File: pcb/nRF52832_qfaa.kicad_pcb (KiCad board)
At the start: 4 copper layers, 41 x 12 mm, 58 parts, among them J2 Conn_02x05_Odd_Even, U1 NRF52832, U2 W25Q32JVZP, U3 TLV75533PDBVR, U4 BQ24078RGTR, X1 32.768kHz, X2 32MHz

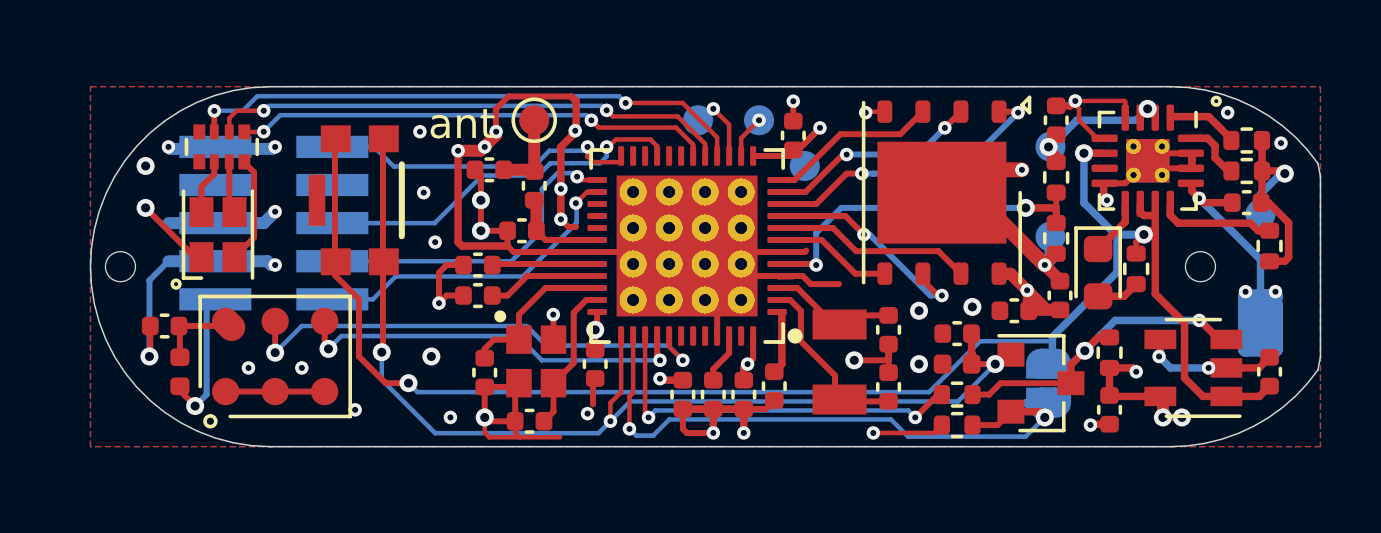
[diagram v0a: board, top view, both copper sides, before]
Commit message: [pcb] v1.2 schematics and PCB, start of the fixture
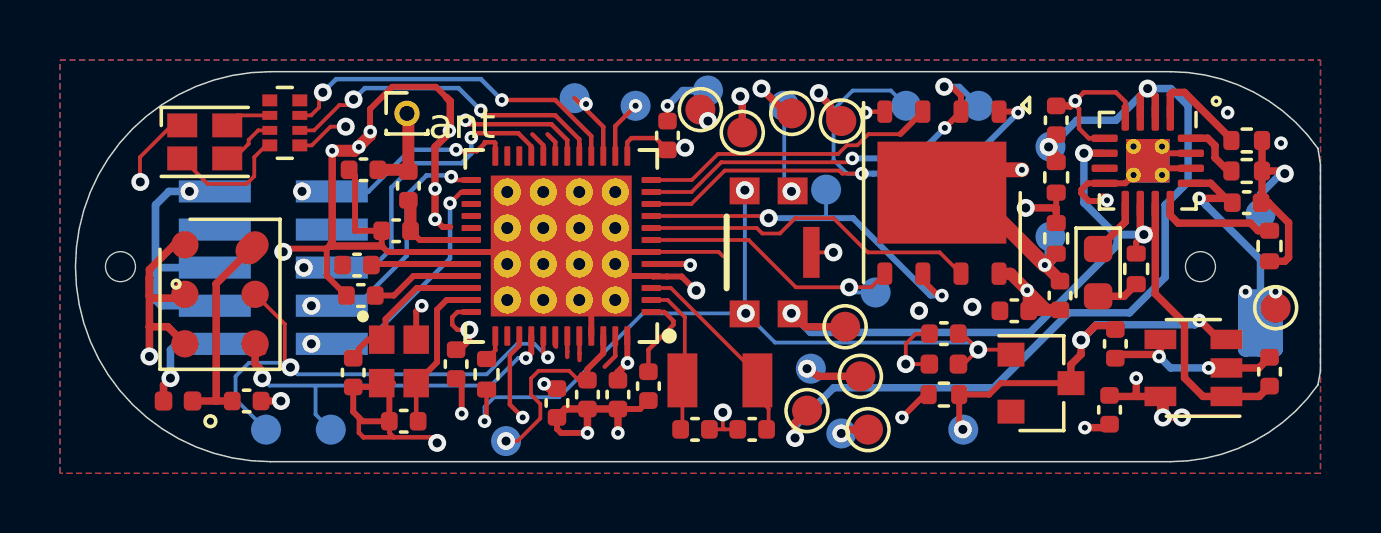
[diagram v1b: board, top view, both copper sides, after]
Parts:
- removed JP1: Jumper_2_Open, Jumper:SolderJumper-2_P1.3mm_Open_RoundedPad1.0x1.5mm
- removed R2: 100K, Resistor_SMD:R_0402_1005Metric
- removed R4: 10K, Resistor_SMD:R_0402_1005Metric
- removed TP5: Antenna, TestPoint:TestPoint_Pad_D1.0mm
- added C23: 100pF, Capacitor_SMD:C_0402_1005Metric, F.Cu at (64.1, 37.9)
- added J1: Conn_01x01_Female, Connector_PinHeader_1.00mm:PinHeader_1x01_P1.00mm_Vertical, F.Cu at (40.5, 30.2)
- added R13: 330, Resistor_SMD:R_0402_1005Metric, F.Cu at (43.2, 38.9)
- added TP10: TestPoint, TestPoint:TestPoint_Pad_D1.0mm, B.Cu at (35.8, 40.8)
- added TP11: TestPoint, TestPoint:TestPoint_Pad_D1.0mm, B.Cu at (43.8, 41.1)
- added TP12: TestPoint, TestPoint:TestPoint_Pad_D1.0mm, B.Cu at (56.1, 36.2)
- added TP13: TestPoint, TestPoint:TestPoint_Pad_D1.0mm, B.Cu at (57.1, 30.0)
- added TP14: TestPoint, TestPoint:TestPoint_Pad_D1.0mm, B.Cu at (59.6, 30.0)
- added TP15: TestPoint, TestPoint:TestPoint_Pad_D1.0mm, B.Cu at (54.5, 32.8)
- added TP16: TestPoint, TestPoint:TestPoint_Pad_D1.0mm, B.Cu at (59.1, 40.8)
- added TP17: TestPoint, TestPoint:TestPoint_Pad_D1.0mm, B.Cu at (54.0, 38.7)
- added TP18: TestPoint, TestPoint:TestPoint_Pad_D1.0mm, B.Cu at (53.1, 30.0)
- added TP19: TestPoint, TestPoint:TestPoint_Pad_D1.0mm, B.Cu at (55.0, 40.9)
- added TP20: TestPoint, TestPoint:TestPoint_Pad_D1.0mm, F.Cu at (50.3, 30.1)
- added TP21: TestPoint, TestPoint:TestPoint_Pad_D1.0mm, F.Cu at (55.0, 30.5)
- added TP22: TestPoint, TestPoint:TestPoint_Pad_D1.0mm, F.Cu at (51.7, 30.9)
- added TP23: TestPoint, TestPoint:TestPoint_Pad_D1.0mm, F.Cu at (53.3, 30.2)
- added TP24: TestPoint, TestPoint:TestPoint_Pad_D1.0mm, F.Cu at (55.1, 37.3)
- added TP25: TestPoint, TestPoint:TestPoint_Pad_D1.0mm, F.Cu at (55.6, 39.0)
- added TP26: TestPoint, TestPoint:TestPoint_Pad_D1.0mm, F.Cu at (69.5, 36.7)
- added TP27: TestPoint, TestPoint:TestPoint_Pad_D1.0mm, F.Cu at (53.8, 40.1)
- added TP28: TestPoint, TestPoint:TestPoint_Pad_D1.0mm, F.Cu at (55.9, 40.8)
- added TP9: TestPoint, TestPoint:TestPoint_Pad_D1.0mm, B.Cu at (38.0, 40.8)
- moved S1 13.7 mm to (52.6, 34.9), turned to -90 degrees
- moved C11 6.60 mm to (50.1, 40.8), turned to 180 degrees
- moved C12 5.63 mm to (52.0, 40.8), turned to 0 degrees
- moved C6 4.64 mm to (42.1, 38.6)
- moved X2 4.58 mm to (40.2, 38.5)
- moved C13 4.38 mm to (38.7, 38.9)
- moved C2 4.20 mm to (45.5, 39.9)
- moved C10 4.19 mm to (40.4, 40.5)
- moved C16 4.19 mm to (49.2, 31.0)
- moved C22 4.19 mm to (39.1, 32.1)
- moved C5 4.19 mm to (47.5, 39.6)
- moved C9 4.19 mm to (48.6, 39.3)
- moved L2 4.19 mm to (40.6, 32.6)
- moved U1 4.19 mm to (45.7, 34.6)
- moved C14 4.19 mm to (40.2, 34.1)
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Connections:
- net /P0.00/XL1 renamed /P0.00/XL1
- net /P0.01/XL2 renamed /P0.01/XL2
- net /P0.18/SWO renamed /P0.18/SWO
- net /P0.21/RESET renamed /P0.21/RESET
- D2 pad 2: DBG_POWER_LATCH -> unconnected-(D2-Pad2)
- J2 pad 7: Net-(J2-Pad7) -> unconnected-(J2-Pad7)
- J2 pad 8: Net-(J2-Pad8) -> unconnected-(J2-Pad8)
- RN1 pad 4: Net-(RN1-Pad4) -> unconnected-(RN1-Pad4)
- RN1 pad 5: Net-(RN1-Pad5) -> unconnected-(RN1-Pad5)
- U1 pad 37: MAIN_BUTTON -> /P0.25
- U1 pad 38: DBG_POWER_LATCH -> unconnected-(U1-Pad38)
- U1 pad 42: Net-(U1-Pad42) -> unconnected-(U1-Pad42)
- U1 pad 43: Net-(U1-Pad43) -> unconnected-(U1-Pad43)
- U1 pad 44: Net-(U1-Pad44) -> unconnected-(U1-Pad44)
- U1 pad 47: Net-(U1-Pad47) -> unconnected-(U1-Pad47)
- U4 pad 7: Net-(U4-Pad7) -> unconnected-(U4-Pad7)
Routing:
- net +BATT: track 5.68 -> 30.8 mm, vias 2 -> 3
- net DBG_POWER_LATCH: track 21.3 -> 0.00 mm, vias 2 -> 0
- net VSS: track 54.5 -> 39.9 mm, vias 3 -> 4
- net /MEM_CS: track 9.94 -> 19.9 mm
- net /SWDCLK: track 11.0 -> 20.9 mm, vias 1 -> 3
- net /SWDIO: track 10.7 -> 20.5 mm, vias 1 -> 3
- net MAIN_BUTTON: track 35.7 -> 27.1 mm, vias 3 -> 4
- net /LED_RED: track 18.9 -> 11.9 mm
- net /MEM_DO: track 7.25 -> 14.1 mm, vias 2 -> 3
- net VCC: track 80.9 -> 86.9 mm, vias 10 -> 12
- net /LED_BLUE: track 17.4 -> 11.6 mm
- net /MEM_DI: track 4.05 -> 9.58 mm, vias 0 -> 1
- net /MEM_CLK: track 7.66 -> 13.0 mm
- net /DEC4: track 1.69 -> 6.90 mm, vias 0 -> 1
- net /MEM_IO3: track 6.76 -> 11.4 mm
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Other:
- board size 41 x 12 mm -> 41.5 x 13 mm
- net class Default removed
- board text added: "Dictofun 1.2"
- board text removed: "Dictofun 1.1"
- board text removed: "dbg on"
